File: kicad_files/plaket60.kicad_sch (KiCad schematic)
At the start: 8 parts, among them J1 SM04B, J2 SWD, U3 XC6206PxxxMR, U4 PRTR5V0U2X

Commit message: j'sais pas
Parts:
- J1: footprint Connector_JST:JST_SH_SM04B-SRSS-TB_1x04-1MP_P1.00mm_Horizontal -> Connector_Molex:Molex_Pico-EZmate_78171-0004_1x04-1MP_P1.20mm_Vertical
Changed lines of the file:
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@@
       (effects (font (size 1.27 1.27)) (justify left))
     )
-    (property "Footprint" "Connector_JST:JST_SH_SM04B-SRSS-TB_1x04-1MP_P1.00mm_Horizontal" (id 2) (at 170.18 22.86 0)
+    (property "Footprint" "Connector_Molex:Molex_Pico-EZmate_78171-0004_1x04-1MP_P1.20mm_Vertical" (id 2) (at 170.18 22.86 0)
       (effects (font (size 1.27 1.27)) hide)
     )
@@
     )
     (path "/b680838b-e6a0-4be0-8ee0-3b59a4379f08"
-      (reference "J1") (unit 1) (value "SM04B") (footprint "Connector_JST:JST_SH_SM04B-SRSS-TB_1x04-1MP_P1.00mm_Horizontal")
+      (reference "J1") (unit 1) (value "SM04B") (footprint "Connector_Molex:Molex_Pico-EZmate_78171-0004_1x04-1MP_P1.20mm_Vertical")
     )
     (path "/43439a45-122d-4862-9414-61a9fa8204f1"

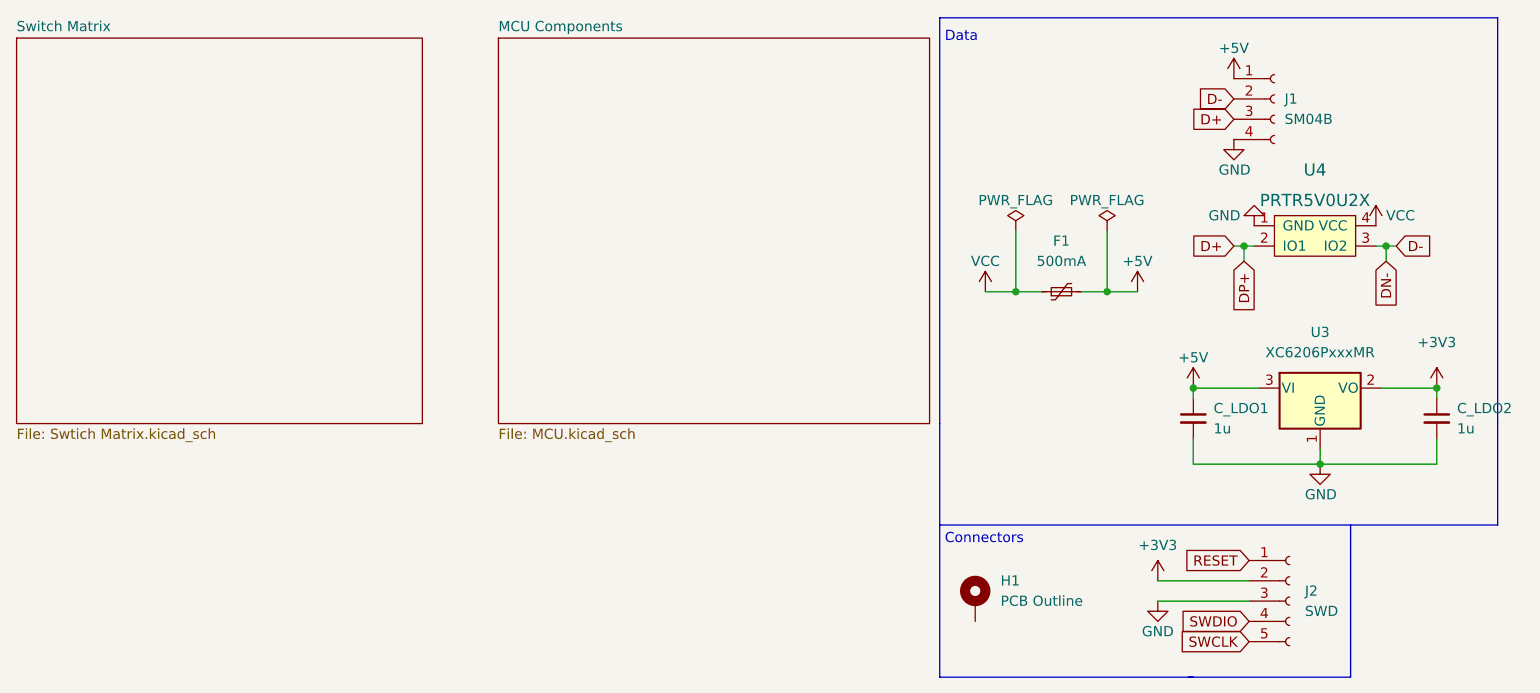
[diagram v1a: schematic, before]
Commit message: double jst
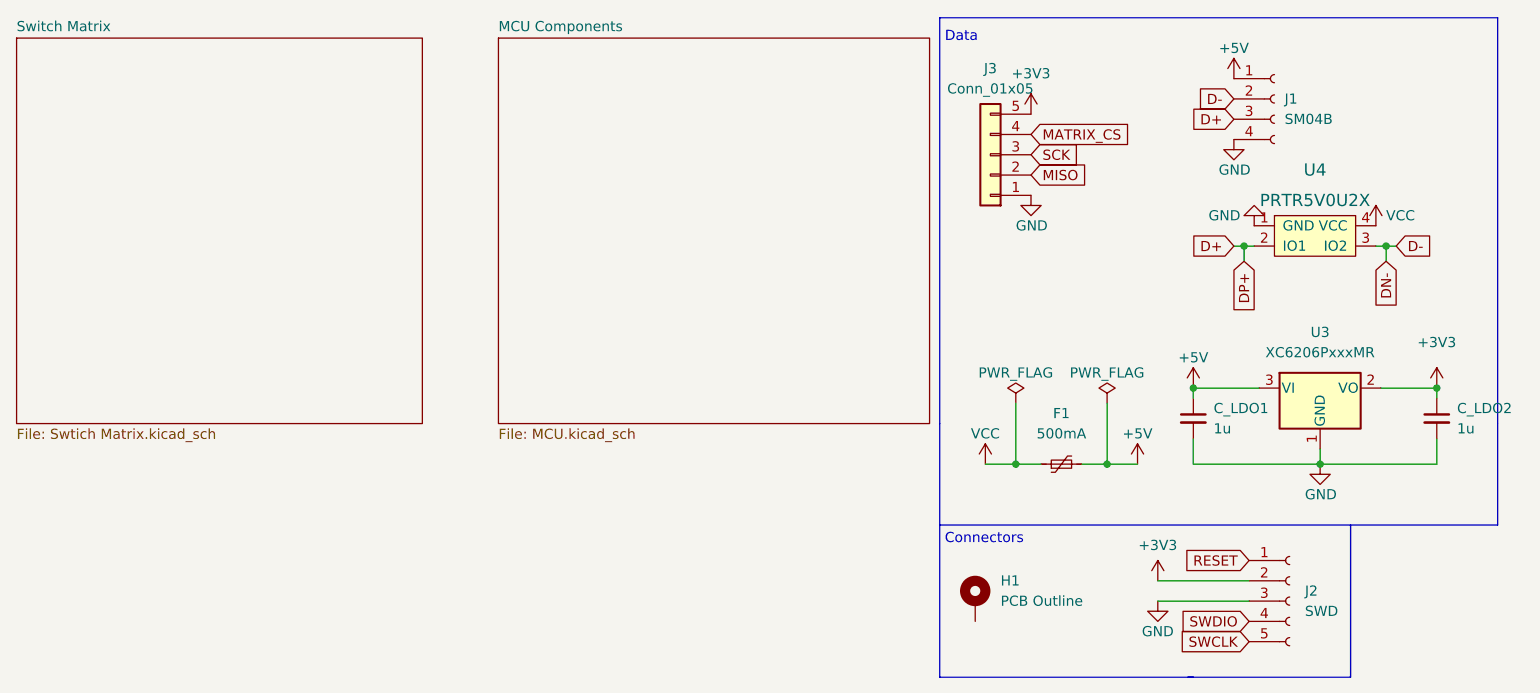
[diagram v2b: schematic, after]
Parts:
- added J3: Conn_01x05, Connector_JST:JST_SH_SM05B-SRSS-TB_1x05-1MP_P1.00mm_Horizontal, symbol Connector_Generic:Conn_01x05
- J1: footprint Connector_Molex:Molex_Pico-EZmate_78171-0004_1x04-1MP_P1.20mm_Vertical -> Connector_JST:JST_SH_SM04B-SRSS-TB_1x04-1MP_P1.00mm_Horizontal
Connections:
- net +3V3: now also J3.5 (Pin_5)
- net GND: now also J3.1 (Pin_1)
- new net MATRIX_CS: J3.4 (Pin_4)
- new net MISO: J3.2 (Pin_2)
- new net SCK: J3.3 (Pin_3)
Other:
- moved on the sheet: F1
